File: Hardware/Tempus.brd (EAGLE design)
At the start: 37 x 50 mm, 36 parts, among them J7 AVR_SPI_PRG_6NS, U1 ATMEGA328P_TQFP, Y1 16MHZ

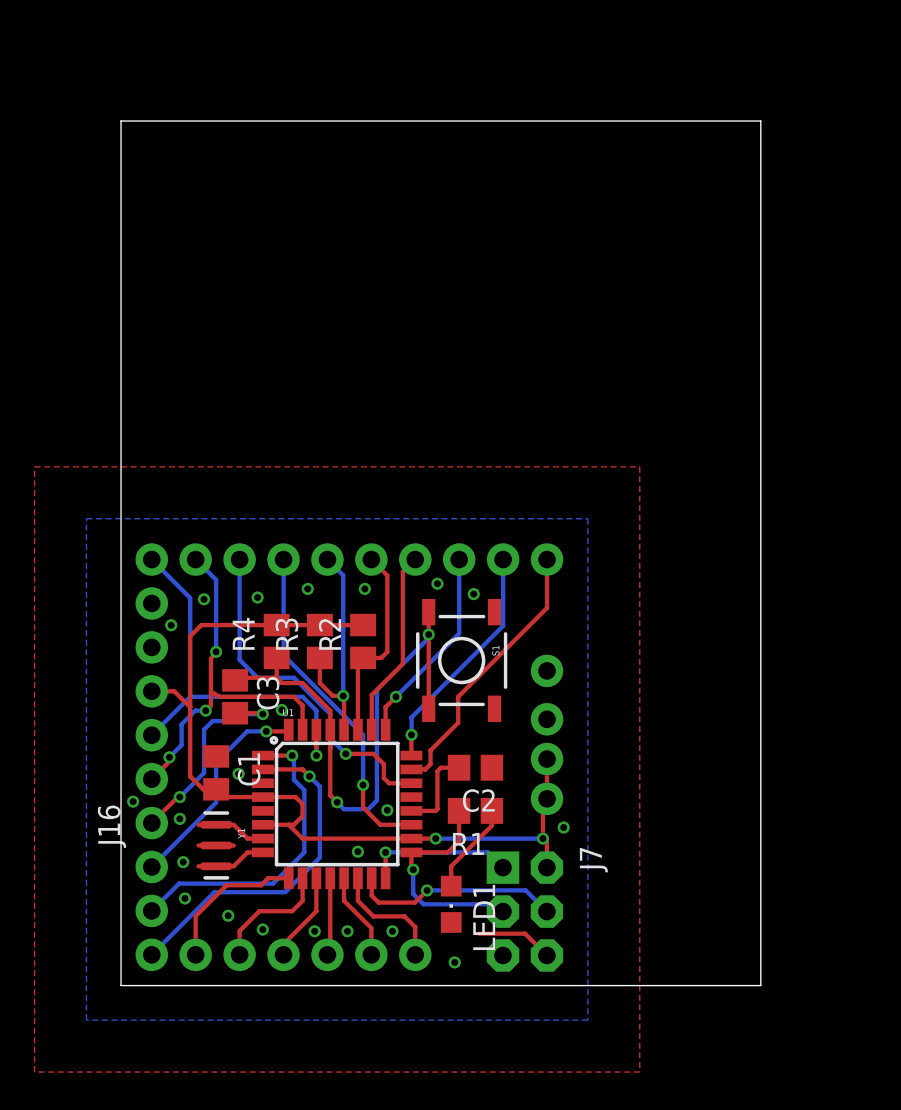
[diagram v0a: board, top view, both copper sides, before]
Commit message: Hardware modifications
Hardware modifications
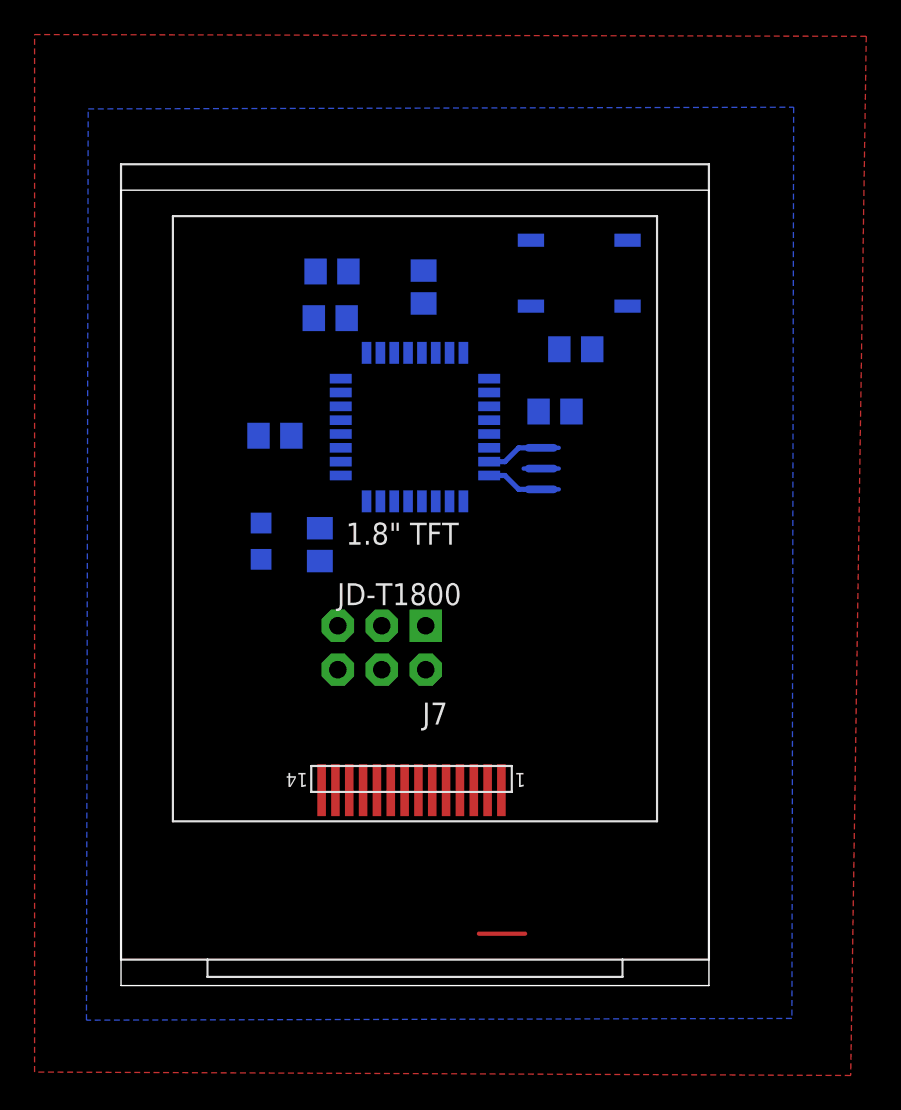
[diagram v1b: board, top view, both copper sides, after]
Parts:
- removed J1, J10, J11, J12, J13, J14, J15, J17, J18, J19, J2, J20, J21, J22, J23, J24, J25, J3, J4, J5, J6, J8, J9: (no value), SparkFun-Connectors:1X01NS-KIT
- removed J16: (no value), SparkFun-Connectors:1X06_NO_SILK
- added U$1: DISP_TFT18, KarlVaello-Displays:TFT18
- moved Y1 28.8 mm to (24.3, 29.9), flipped to the bottom
- moved C1 28.7 mm to (25.1, 33.2), flipped to the bottom, turned to 0 degrees
- moved C3 28.1 mm to (26.3, 36.8), flipped to the bottom, turned to 0 degrees
- moved LED1 23.7 mm to (8.10, 25.7), flipped to the bottom, turned to 0 degrees
- moved S1 23.4 mm to (26.5, 41.2), flipped to the bottom, turned to 0 degrees
- moved C2 22.4 mm to (8.90, 31.8), flipped to the bottom
- moved U1 22.3 mm to (17.0, 32.3), flipped to the bottom
- moved R4 22.2 mm to (17.5, 40.4), flipped to the bottom
- moved R3 21.4 mm to (12.2, 41.3), flipped to the bottom, turned to 0 degrees
- moved R2 18.8 mm to (12.1, 38.6), flipped to the bottom, turned to 0 degrees
- moved R1 17.8 mm to (11.5, 25.5), flipped to the bottom, turned to 90 degrees
- moved J7 17.4 mm to (15.1, 19.5), turned to 180 degrees
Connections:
- net A0: no longer J1.1
- net A1: no longer J2.1
- net A2: no longer J3.1
- net A3: no longer J17.1
- net A4: no longer J20.1
- net A5: no longer J21.1
- net A6: no longer J18.1
- net A7: no longer J19.1
- net D10: no longer J6.1
- net D2: no longer J11.1
- net D3: no longer J12.1
- net D4: no longer J13.1
- net D5: no longer J14.1
- net D6: no longer J15.1
- net D7: no longer J8.1
- net D8: no longer J4.1
- net D9: no longer J5.1
- net DTR: no longer J16.1
- net GND: no longer J16.5, J16.6, J24.1, J25.1
- net RXI: no longer J16.3, J9.1
- net TXO: no longer J10.1, J16.2
- net VCC: no longer J16.4, J22.1, J23.1
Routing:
- net VCC: track 52.8 -> 0.00 mm, vias 2 -> 0
- net RESET: track 33.5 -> 0.00 mm, vias 2 -> 0
- net RXI: track 23.7 -> 0.00 mm, vias 1 -> 0
- net TXO: track 22.1 -> 0.00 mm, vias 3 -> 0
- net A7: track 20.0 -> 0.00 mm, vias 1 -> 0
- net D4: track 19.9 -> 0.00 mm, vias 1 -> 0
- net A6: track 19.5 -> 0.00 mm, vias 1 -> 0
- net D3: track 17.8 -> 0.00 mm, vias 1 -> 0
- net A0: track 15.9 -> 0.00 mm
- net A1: track 13.5 -> 0.00 mm, vias 1 -> 0
- net A5: track 13.4 -> 0.00 mm, vias 1 -> 0
- net SCK: track 12.8 -> 0.00 mm, vias 1 -> 0
- net D2: track 12.6 -> 0.00 mm, vias 1 -> 0
- net DTR: track 12.1 -> 0.00 mm, vias 2 -> 0
- net MOSI: track 12.1 -> 0.00 mm, vias 1 -> 0
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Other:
- board size 37 x 50 mm -> 34 x 46 mm
